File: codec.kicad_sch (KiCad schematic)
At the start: 10 parts, among them U15 TAC5111IRGER, U17 LM321

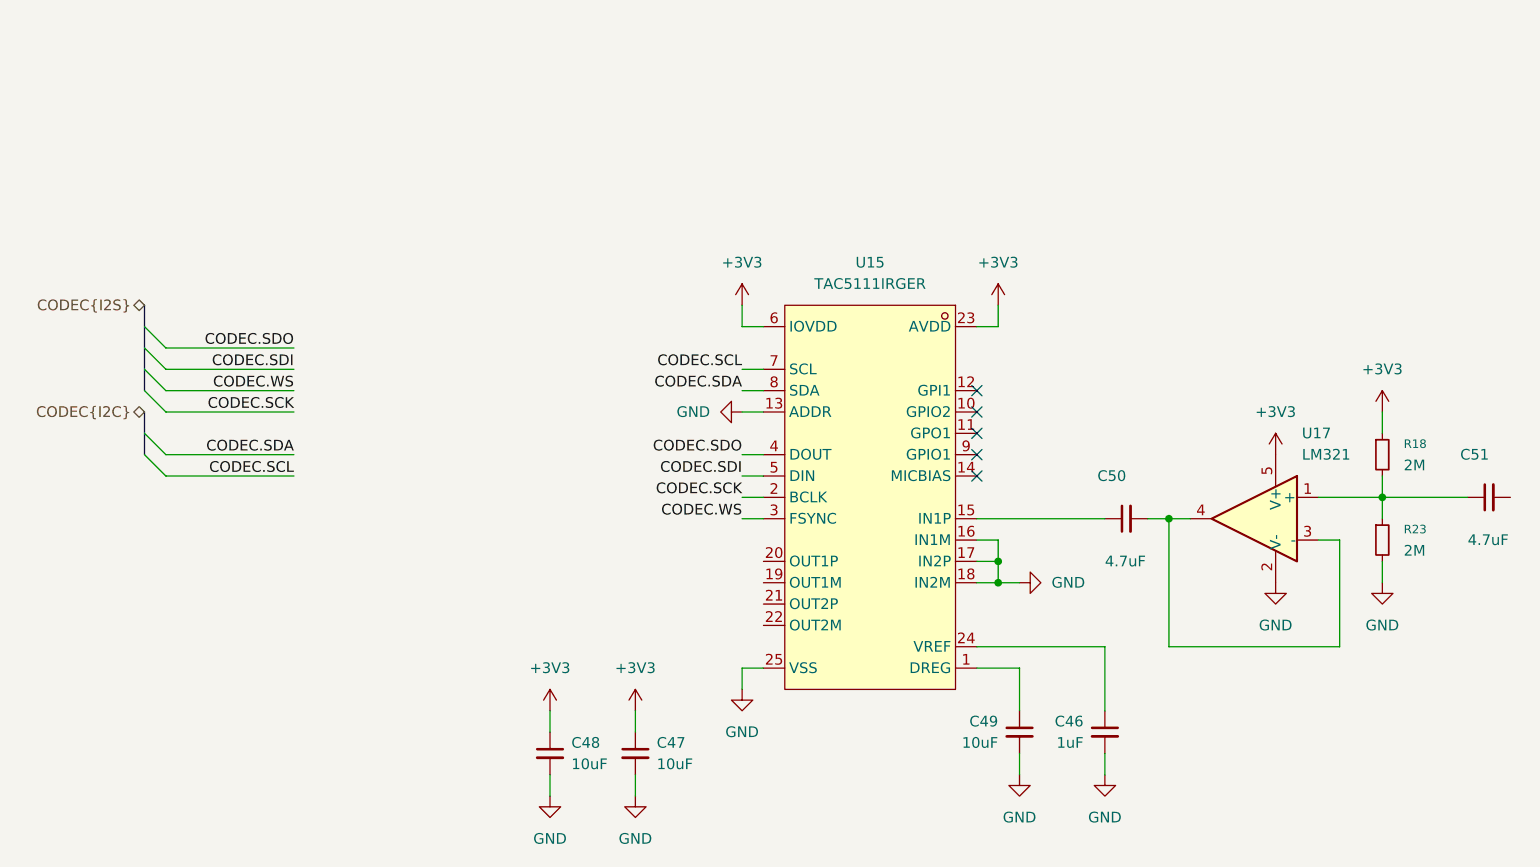
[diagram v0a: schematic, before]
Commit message: Finalize input buffer and filtering
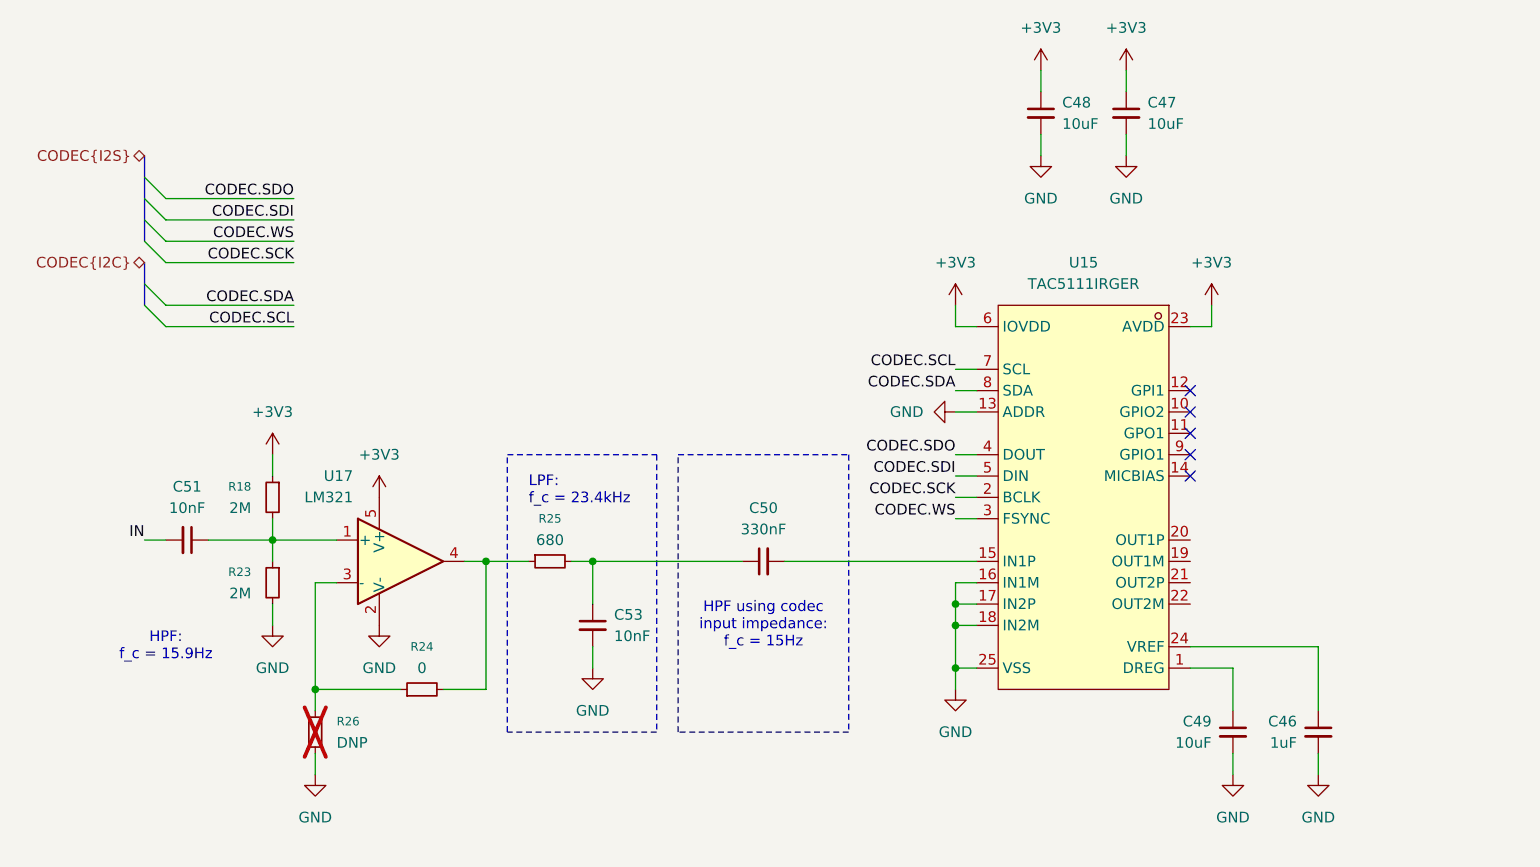
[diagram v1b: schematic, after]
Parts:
- added C53: 10nF, Capacitor_SMD:C_0603_1608Metric, symbol Device:C_Small
- added R24: 0, Resistor_SMD:R_0402_1005Metric, symbol Device:R_Small
- added R25: 680, Resistor_SMD:R_0402_1005Metric, symbol Device:R_Small
- added R26: DNP, Resistor_SMD:R_0402_1005Metric, symbol Device:R_Small
- C50: value 4.7uF -> 330nF; footprint Capacitor_SMD:C_0402_1005Metric -> Resistor_SMD:R_1206_3216Metric; Dielectric (none) -> C0G; LCSC C23733 -> C3837965; Voltage (none) -> 25
- C51: value 4.7uF -> 10nF; footprint Capacitor_SMD:C_0402_1005Metric -> Capacitor_SMD:C_0603_1608Metric; LCSC C23733 -> C76599; Voltage (none) -> 50
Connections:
- net GND: now also C53.2, R26.1
- net at U15.15 (IN1P): now also C50.2; no longer C50.1
- net IN: now reaches C51.2
- new net: R24.1, R26.2, U17.3 (-)
- new net: R24.2, R25.1, U17.4
- new net: C50.1, C53.1, R25.2
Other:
- note added: "HPF using codec input impedance: f_c = 15Hz"
- note added: "HPF: f_c = 15.9Hz"
- note added: "LPF: f_c = 23.4kHz"
- moved on the sheet: C46, C47, C48, C49, R18, R23, U15, U17
